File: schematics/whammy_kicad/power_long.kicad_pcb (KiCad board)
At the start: 2 copper layers, 31 parts, among them U2 L7915, U3 L7815

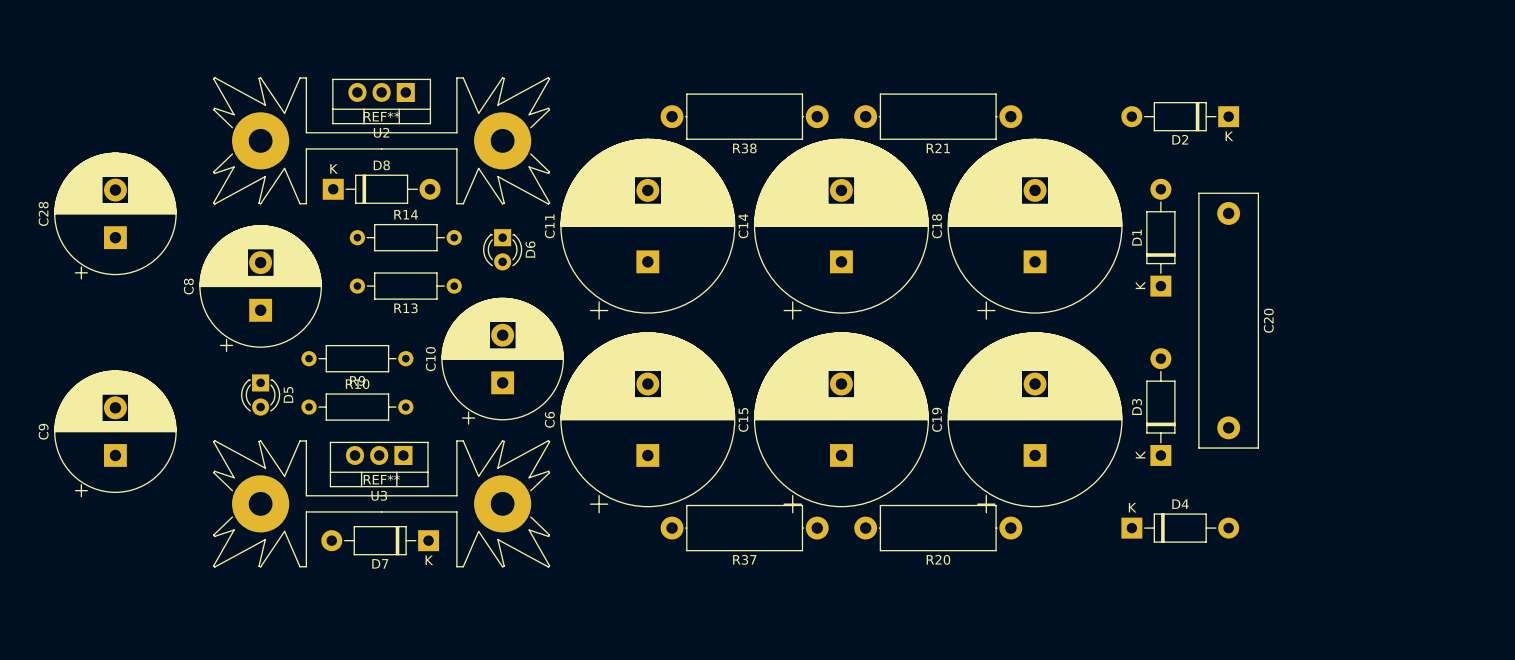
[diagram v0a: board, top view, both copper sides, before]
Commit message: Final version
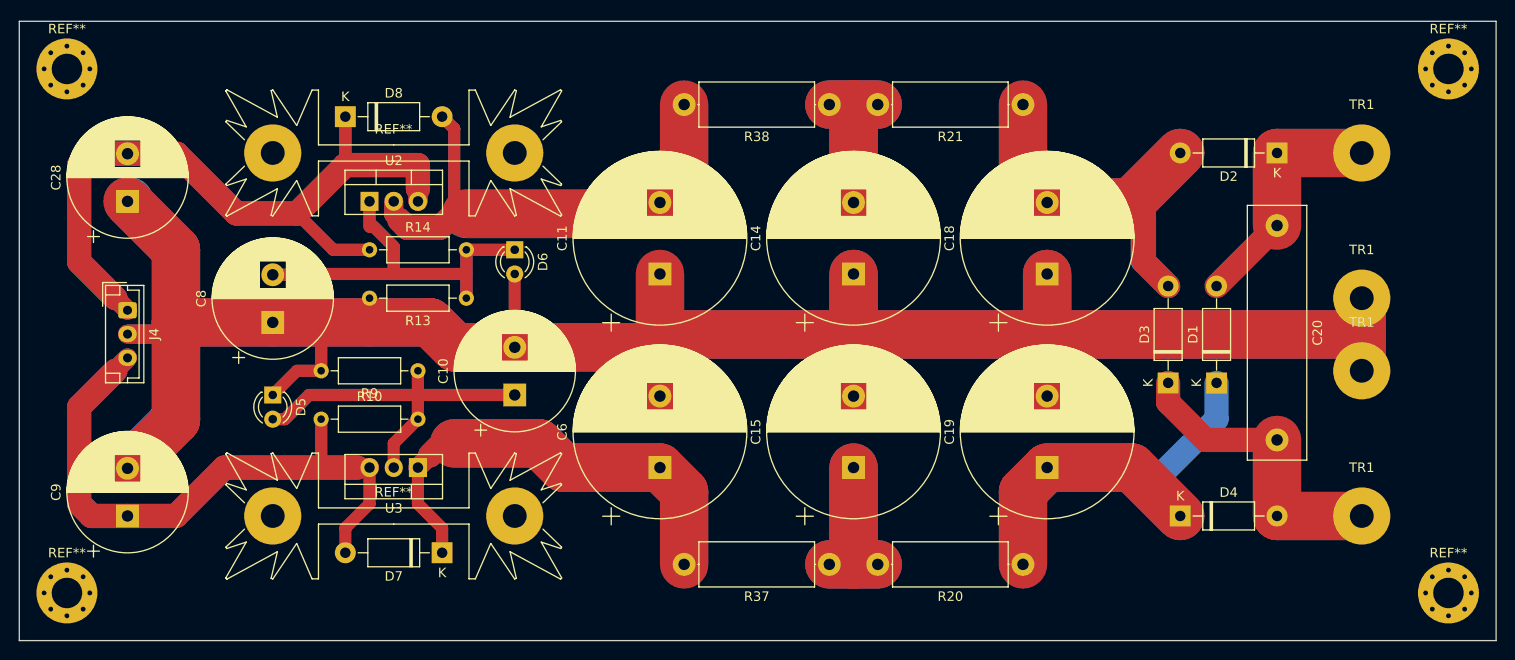
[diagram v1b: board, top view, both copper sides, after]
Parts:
- removed the REF** at (113.0, 120.7)
- removed the REF** at (113.0, 82.5)
- added J4: Conn_01x03, Connector_JST:JST_EH_B3B-EH-A_1x03_P2.50mm_Vertical, F.Cu at (86.4, 100.3)
- added REF**: MountingHole_3.2mm_M3_Pad_Via, MountingHole:MountingHole_3.2mm_M3_Pad_Via, F.Cu at (80.0, 75.0)
- added REF**: MountingHole_3.2mm_M3_Pad_Via, MountingHole:MountingHole_3.2mm_M3_Pad_Via, F.Cu at (80.0, 130.0)
- added REF**: MountingHole_3.2mm_M3_Pad_Via, MountingHole:MountingHole_3.2mm_M3_Pad_Via, F.Cu at (225.0, 130.0)
- added REF**: MountingHole_3.2mm_M3_Pad_Via, MountingHole:MountingHole_3.2mm_M3_Pad_Via, F.Cu at (225.0, 75.0)
- added REF**: Heatsink_Fischer_SK104-STC-STIC_35x13mm_2xDrill2.5mm, Heatsink:Heatsink_Fischer_SK104-STC-STIC_35x13mm_2xDrill2.5mm, F.Cu at (114.3, 121.9)
- added REF**: Heatsink_Fischer_SK104-STC-STIC_35x13mm_2xDrill2.5mm, Heatsink:Heatsink_Fischer_SK104-STC-STIC_35x13mm_2xDrill2.5mm, F.Cu at (114.3, 83.8)
- added TR1: SolderWirePad_1x01_Drill2.5mm, Connector_Wire:SolderWirePad_1x01_Drill2.5mm, F.Cu at (215.9, 99.1)
- added TR1: SolderWirePad_1x01_Drill2.5mm, Connector_Wire:SolderWirePad_1x01_Drill2.5mm, F.Cu at (215.9, 106.7)
- added TR1: SolderWirePad_1x01_Drill2.5mm, Connector_Wire:SolderWirePad_1x01_Drill2.5mm, F.Cu at (215.9, 121.9)
- added TR1: SolderWirePad_1x01_Drill2.5mm, Connector_Wire:SolderWirePad_1x01_Drill2.5mm, F.Cu at (215.9, 83.8)
- C10, C28, C8, C9: value 220uF/25V -> 220uF/50V
- moved U2 12.0 mm to (111.8, 88.9), turned to 0 degrees
- moved D1 11.7 mm to (200.7, 108.0)
- moved D8 7.73 mm to (109.2, 80.0)
- moved D3 7.66 mm to (195.6, 108.0)
- moved C9 6.48 mm to (86.4, 121.9)
- moved D2 6.35 mm to (207.0, 83.8)
- moved C20 5.24 mm to (207.0, 91.4)
- moved D4 5.24 mm to (196.8, 121.9)
- moved R20 4.02 mm to (180.3, 127.0)
- moved R37 4.02 mm to (160.0, 127.0)
- moved C28 4.02 mm to (86.4, 88.9)
- moved U3 1.98 mm to (116.8, 116.8)
- moved D7 1.91 mm to (119.4, 125.8)
- moved C15 1.80 mm to (162.6, 116.8)
- moved C6 1.80 mm to (142.2, 116.8)
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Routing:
- net GND: track 0.00 -> 435.7 mm
- net -15V: track 0.00 -> 152.4 mm
- net +15V: track 0.00 -> 121.2 mm
- net Net-(C11-Pad2): track 0.00 -> 95.0 mm
- net Net-(C6-Pad1): track 0.00 -> 76.2 mm
- net Net-(C8-Pad2): track 0.00 -> 73.4 mm
- net Net-(C10-Pad1): track 0.00 -> 69.2 mm
- net Net-(C18-Pad2): track 0.00 -> 64.4 mm
- net Net-(C19-Pad1): track 0.00 -> 57.4 mm
- net Net-(C20-Pad2): track 0.00 -> 32.0 mm
- net Net-(C14-Pad2): track 0.00 -> 30.7 mm
- net Net-(C15-Pad1): track 0.00 -> 30.5 mm
- net Net-(C20-Pad1): track 0.00 -> 25.5 mm
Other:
- board outline added: 155 x 65 mm
- net class Power added: clearance 0.5, trace_width 0.25, via_dia 0.8, via_drill 0.4
